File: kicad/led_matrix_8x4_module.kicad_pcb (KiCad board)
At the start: 2 copper layers, 96.1 x 98.4 mm, 64 parts, among them J1 Conn_01x04, J2 Conn_01x02_Female, J3 Conn_01x04_Female, J4 DIP_SOCKET_02x08, Q1 PN2222A, Q2 PN2222A, Q3 PN2222A, Q4 PN2222A, Q5 PN2222A, Q6 PN2222A, Q7 PN2222A, Q8 PN2222A, U1 74HC595

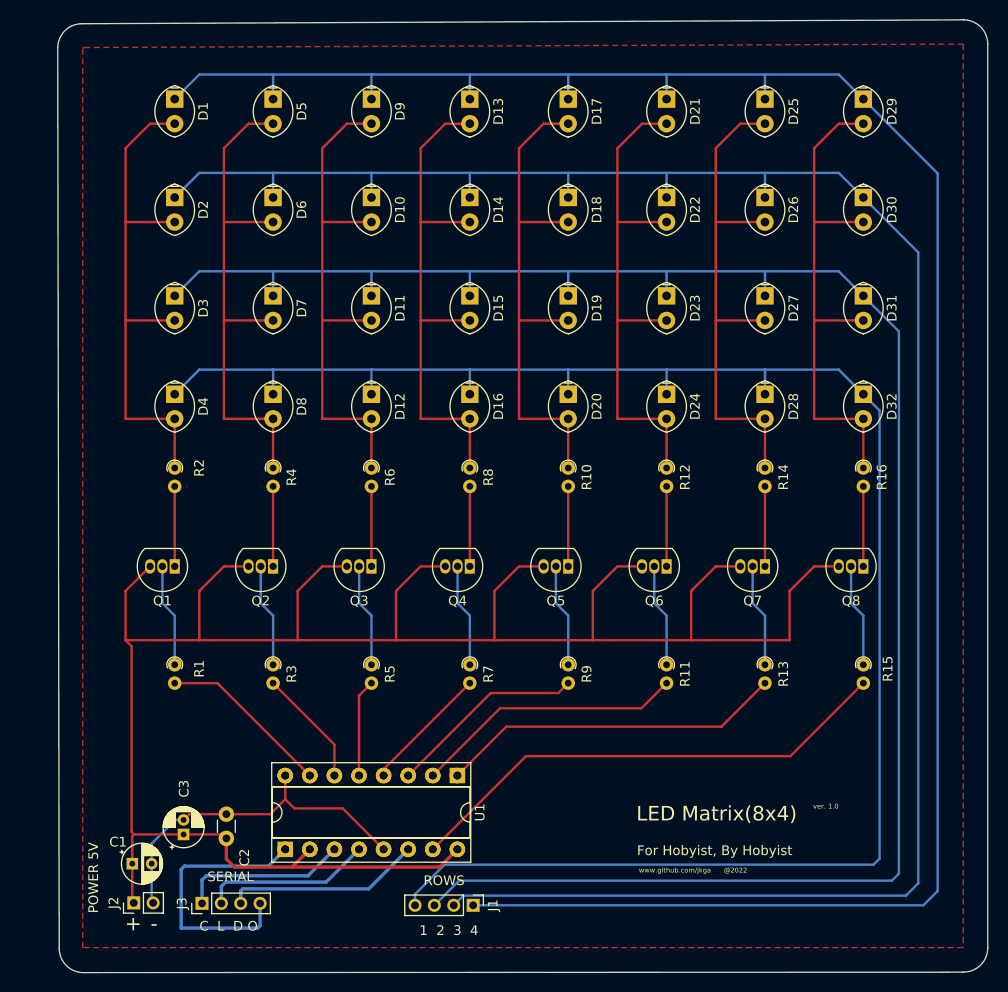
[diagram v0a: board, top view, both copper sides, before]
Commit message: release: v1.1
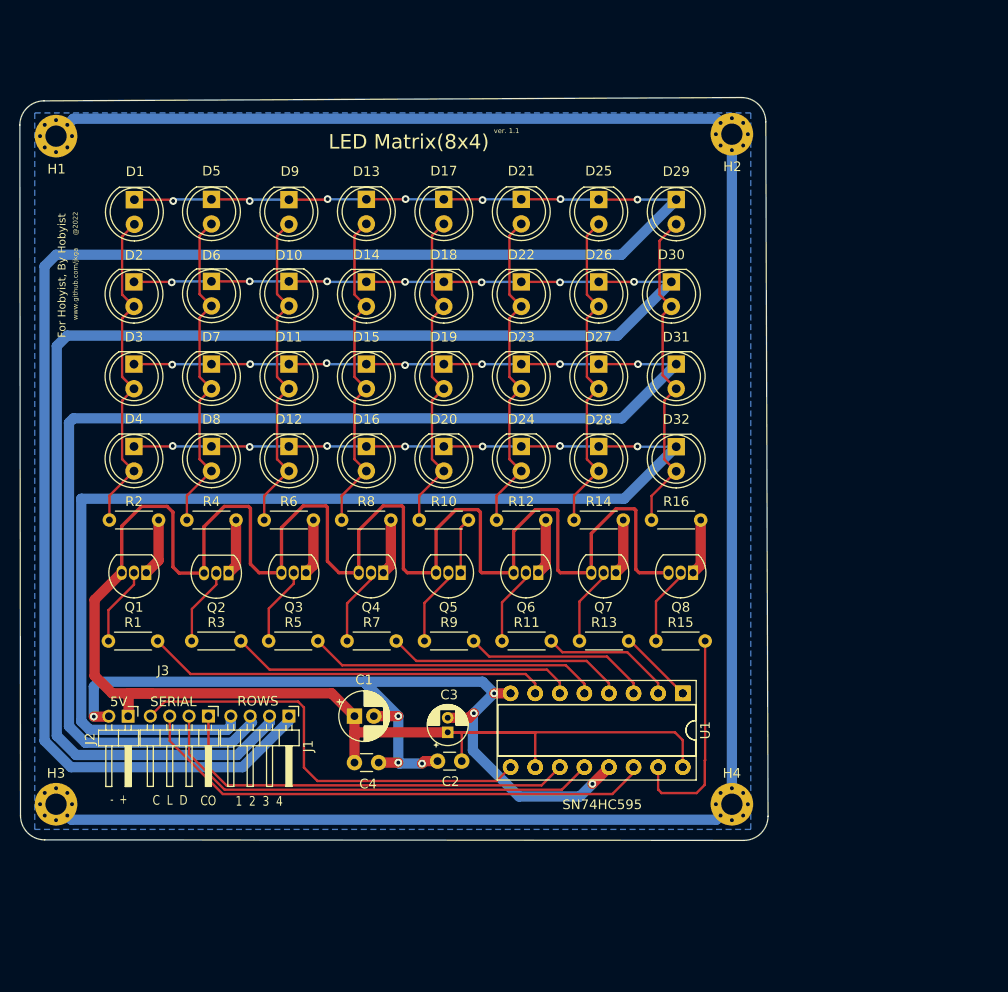
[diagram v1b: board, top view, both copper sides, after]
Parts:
- added C4: 0.1uf, Capacitor_THT:C_Disc_D3.0mm_W1.6mm_P2.50mm, F.Cu at (128.5, 118.4)
- added H1: MountingHole, MountingHole:MountingHole_2.2mm_M2_Pad_Via, F.Cu at (97.7, 53.7)
- added H2: MountingHole, MountingHole:MountingHole_2.2mm_M2_Pad_Via, F.Cu at (167.5, 53.5)
- added H3: MountingHole, MountingHole:MountingHole_2.2mm_M2_Pad_Via, F.Cu at (97.7, 122.7)
- added H4: MountingHole, MountingHole:MountingHole_2.2mm_M2_Pad_Via, F.Cu at (167.5, 122.7)
- C1: value 33uf -> 100uf; footprint Capacitor_THT:CP_Radial_D4.0mm_P2.00mm -> Capacitor_THT:CP_Radial_D5.0mm_P2.00mm
- C3: value 0.1uf -> 33uf
- D1, D10, D11, D12, D13, D14, D15, D16, D17, D18, D19, D2, D20, D21, D22, D23, D24, D25, D26, D27, D28, D29, D3, D30, D31, D32, D4, D5, D6, D7, D8, D9: footprint LED_THT:LED_Oval_W5.2mm_H3.8mm -> LED_THT:LED_D5.0mm
- J1, J3: footprint Connector_PinHeader_2.00mm:PinHeader_1x04_P2.00mm_Vertical -> Connector_PinHeader_2.00mm:PinHeader_1x04_P2.00mm_Horizontal
- J2: footprint Connector_PinHeader_2.00mm:PinHeader_1x02_P2.00mm_Vertical -> Connector_PinHeader_2.00mm:PinHeader_1x02_P2.00mm_Horizontal
- R1, R10, R11, R12, R13, R14, R15, R16, R2, R3, R4, R5, R6, R7, R8, R9: footprint Resistor_THT:R_Axial_DIN0204_L3.6mm_D1.6mm_P1.90mm_Vertical -> Resistor_THT:R_Axial_DIN0204_L3.6mm_D1.6mm_P5.08mm_Horizontal
- moved J4 44.1 mm to (162.4, 111.3), turned to -90 degrees
- moved C3 29.2 mm to (138.1, 115.3)
- moved C1 27.5 mm to (128.5, 113.6)
- moved J1 27.3 mm to (121.7, 113.6)
- moved C2 25.6 mm to (139.6, 118.3), turned to 180 degrees
- moved U1 24.8 mm to (162.4, 111.3)
- moved R16 22.5 mm to (159.2, 93.4), turned to 0 degrees
- moved D29 21.9 mm to (161.7, 60.3)
- moved D30 21.7 mm to (161.2, 68.8)
- moved R15 21.6 mm to (159.6, 105.8), turned to 0 degrees
- moved D31 20.6 mm to (161.7, 77.3)
- moved R14 20.4 mm to (151.2, 93.4), turned to 0 degrees
- moved D32 20.1 mm to (161.7, 85.8)
- moved D25 20.1 mm to (153.7, 60.3)
- moved J3 19.4 mm to (113.4, 113.6), turned to -90 degrees
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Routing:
- net (no net): track 0.00 -> 236.3 mm
- net GNDREF: track 36.6 -> 94.4 mm, vias 0 -> 7
- net DataPin: track 20.4 -> 54.2 mm
- net LatchPin: track 17.6 -> 47.2 mm
- net Pin8: track 51.6 -> 22.5 mm
- net Net-(D12-Pad1): track 187.8 -> 159.9 mm, vias 0 -> 7
- net Pin7: track 35.7 -> 7.83 mm
- net ClockPin: track 17.4 -> 43.1 mm
- net Net-(D11-Pad1): track 199.0 -> 173.3 mm, vias 0 -> 7
- net Pin1: track 17.9 -> 41.8 mm
- net Pin2: track 12.2 -> 35.8 mm
- net Net-(D10-Pad1): track 210.6 -> 187.0 mm, vias 0 -> 7
- net Pin3: track 10.1 -> 30.3 mm
- net Net-(D10-Pad2): track 54.4 -> 34.6 mm
- net Net-(D1-Pad2): track 54.4 -> 34.7 mm
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- added copper zone on B.Cu, net GNDREF
- removed copper zone on F.Cu, net (none)
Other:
- board size 96.1 x 98.4 mm -> 77.3 x 76.7 mm
- board text added: "- +"
- board text added: "5V"
- board text added: "C L D"
- board text added: "CO"
- board text added: "SN74HC595"
- board text added: "ver. 1.1"
- board text removed: "+"
- board text removed: "-"
- board text removed: "C L D O"
- board text removed: "POWER 5V"
- board text removed: "ver. 1.0"
